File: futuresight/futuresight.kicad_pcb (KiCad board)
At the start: 2 copper layers, 119.5 x 60 mm, 40 parts, among them J1 Conn_02x13_Odd_Even, J2 Conn_02x13_Odd_Even, J3 Conn_01x02, Q1 AO3401A, SW1 SW_Push, U1 TPS54360DDA

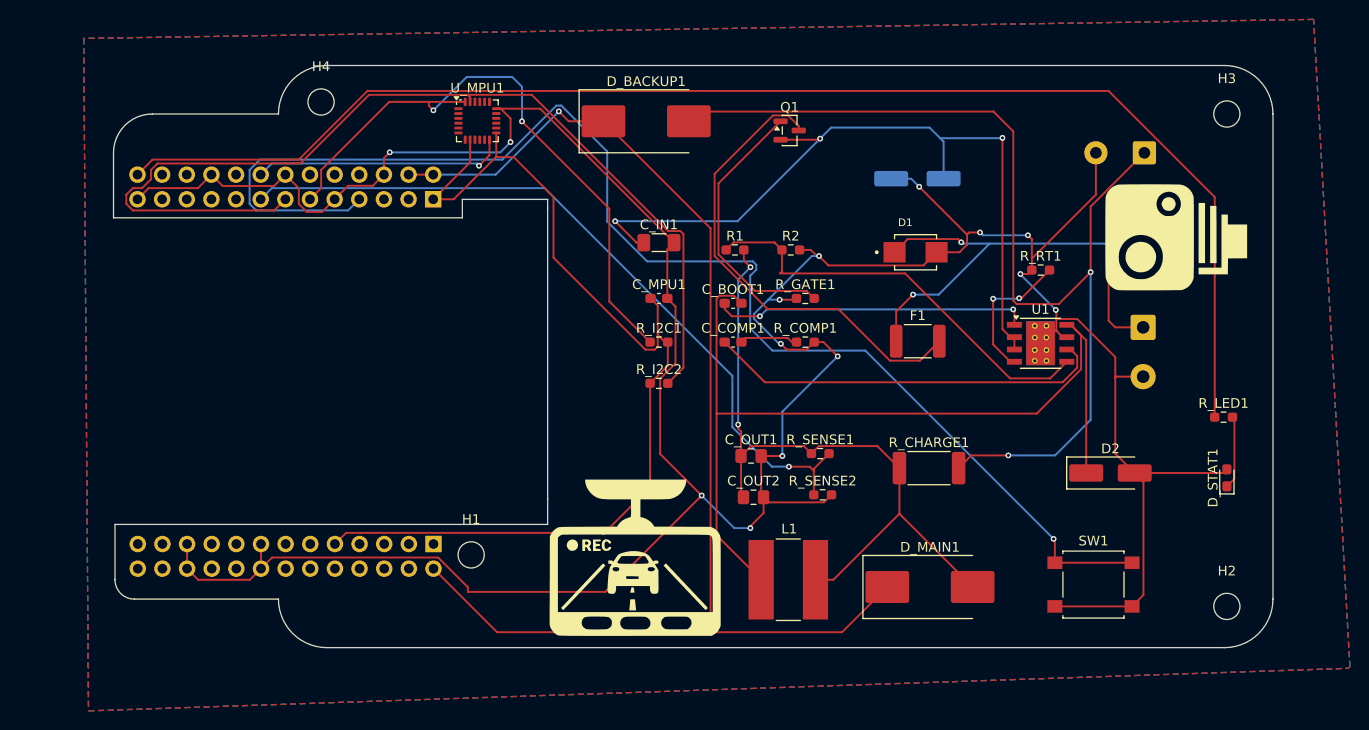
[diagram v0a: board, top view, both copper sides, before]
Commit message: updated -- pcb CAD firmware
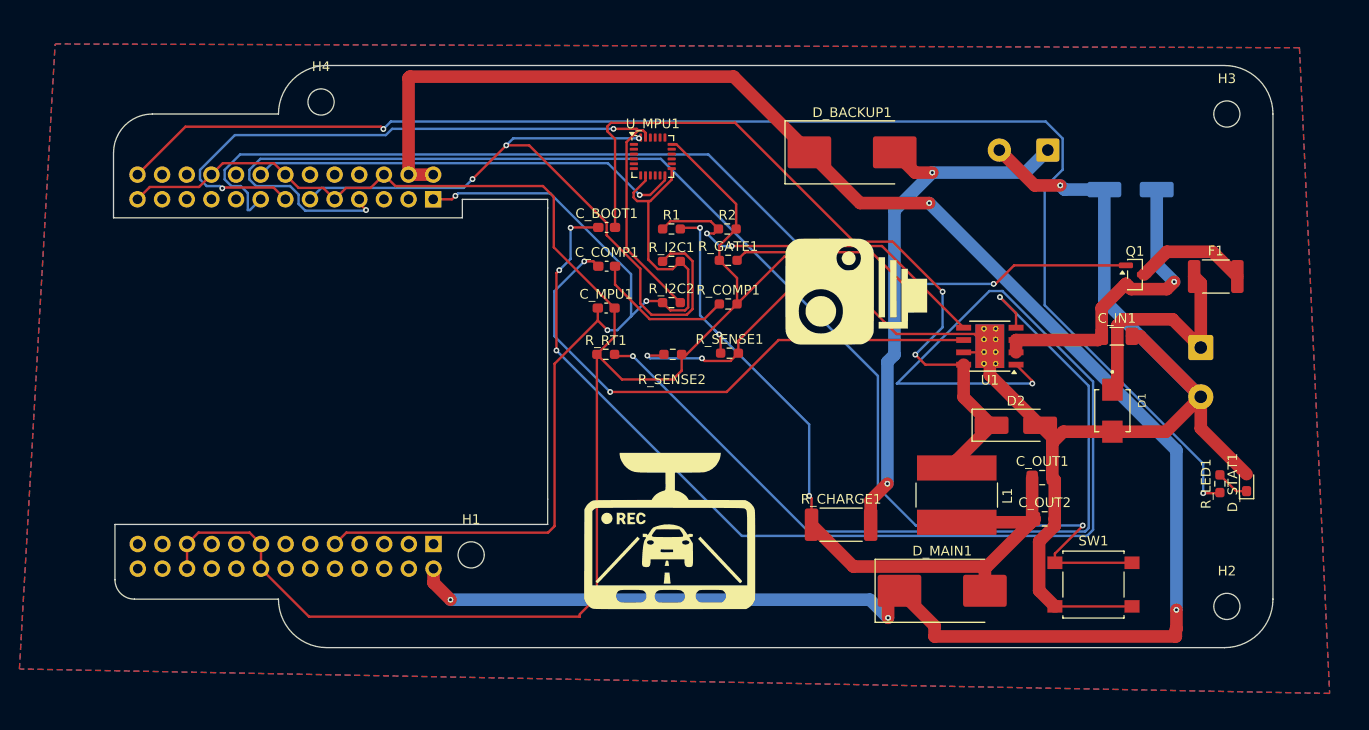
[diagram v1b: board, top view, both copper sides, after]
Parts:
- moved C_IN1 48.2 mm to (175.2, 93.4)
- moved R_RT1 45.7 mm to (122.5, 95.3)
- moved Q1 38.6 mm to (177.0, 87.0)
- moved G*** 33.5 mm to (148.4, 88.6)
- moved F1 31.4 mm to (185.4, 87.2)
- moved C_OUT1 30.1 mm to (167.5, 108.0)
- moved C_OUT2 30.1 mm to (167.7, 112.2)
- moved D1 26.0 mm to (174.7, 101.1), turned to -90 degrees
- moved C_IN2 22.0 mm to (176.6, 78.3)
- moved D_BACKUP1 21.5 mm to (147.9, 74.5)
- moved R_SENSE2 21.2 mm to (129.4, 95.3)
- moved L1 19.4 mm to (158.7, 109.8), turned to -90 degrees
- moved U_MPU1 18.5 mm to (127.3, 74.9)
- moved C_BOOT1 15.2 mm to (122.6, 82.2)
- moved C_COMP1 15.2 mm to (122.6, 86.2)
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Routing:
- net C_boot_1: track 32.6 -> 139.5 mm, vias 2 -> 4
- net +5V_DUO: track 131.9 -> 211.0 mm, vias 1 -> 4
- net Net-(U1-RT/CLK): track 14.7 -> 88.0 mm
- net Net-(D_BACKUP1-A): track 107.1 -> 56.5 mm
- net +12V_PROT: track 79.3 -> 32.5 mm, vias 3 -> 1
- net MOSFET_Drain: track 49.0 -> 11.6 mm
- net +12V_RAW: track 50.2 -> 24.5 mm, vias 3 -> 0
- net I2C1_SCL: track 103.2 -> 79.6 mm, vias 0 -> 2
- net PWR_LOSS_GPIO: track 77.5 -> 98.4 mm, vias 1 -> 3
- net INT: track 26.2 -> 44.6 mm
- net GND: track 352.0 -> 333.7 mm, vias 14 -> 1
- net Net-(U1-COMP): track 41.2 -> 57.4 mm, vias 0 -> 2
- net U1_pin8: track 94.7 -> 79.0 mm, vias 0 -> 2
- net Net-(Q1-G): track 28.1 -> 43.5 mm, vias 0 -> 2
- net I2C1_SDA: track 65.1 -> 74.9 mm, vias 2 -> 3
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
